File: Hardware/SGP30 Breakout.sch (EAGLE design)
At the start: 26 parts, among them J3 PTH, Q1 MOSFET-NCH-BSS138, Q2 MOSFET-NCH-BSS138, U1 SGP30, U2 MIC5504

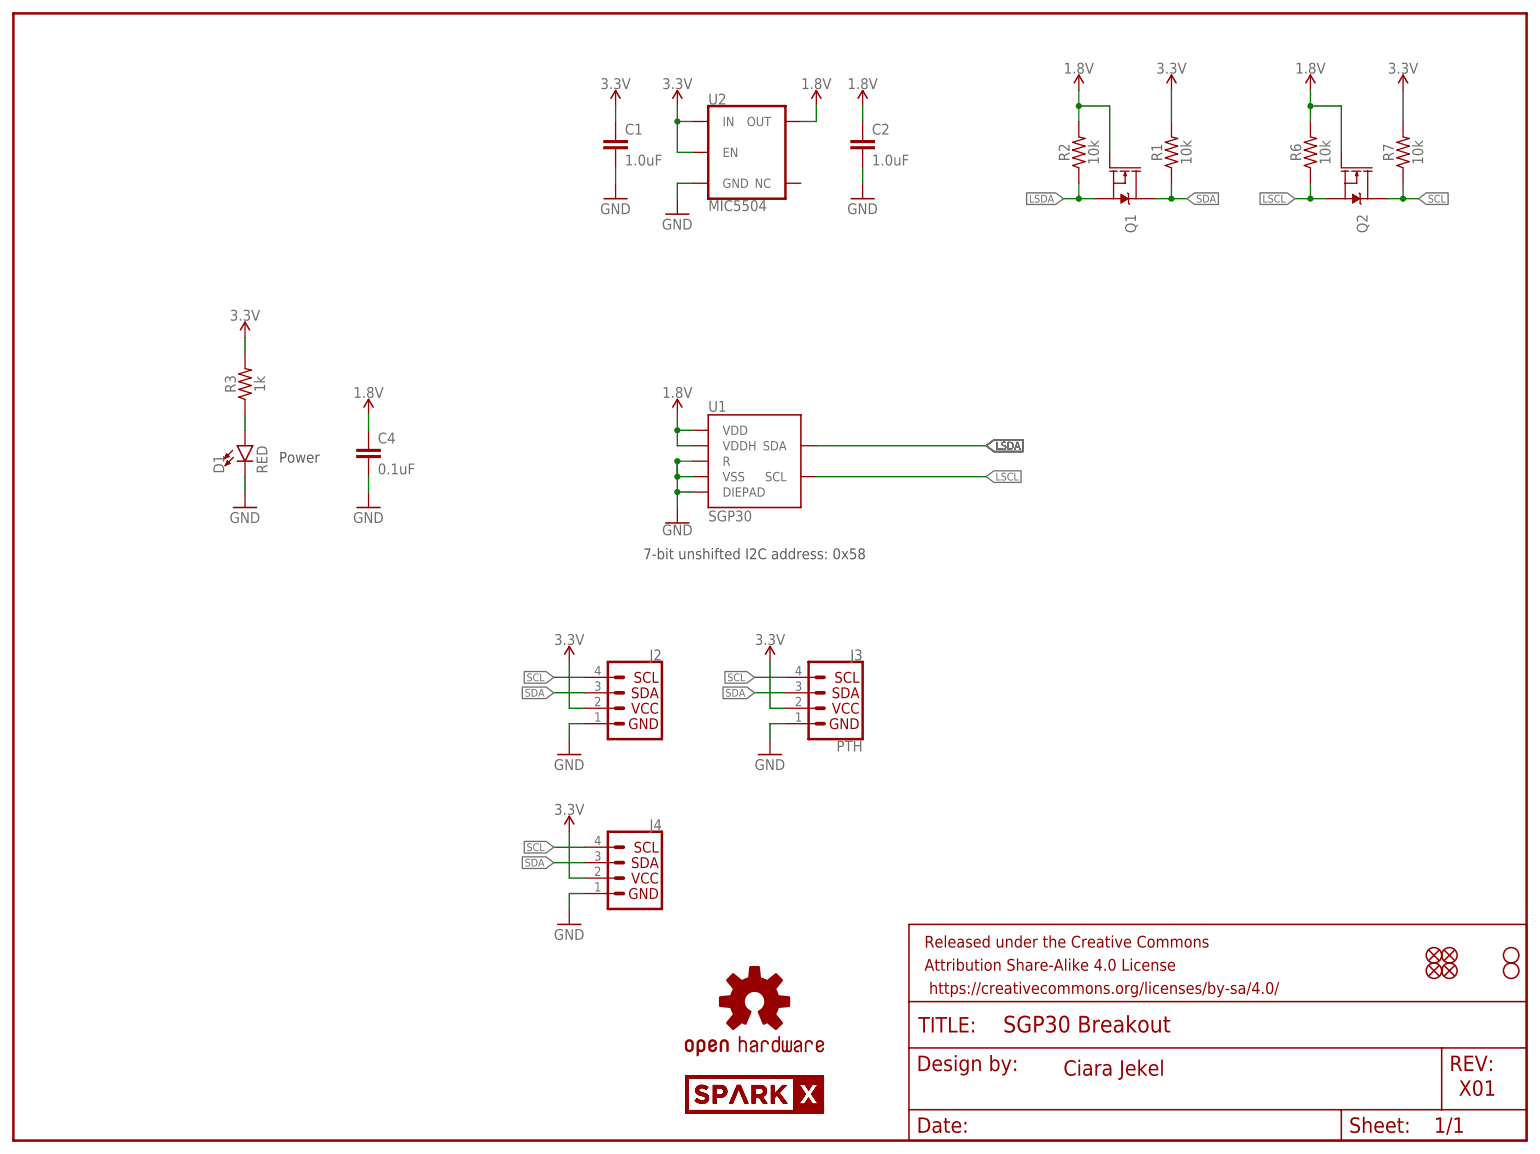
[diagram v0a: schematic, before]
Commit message: added section labels
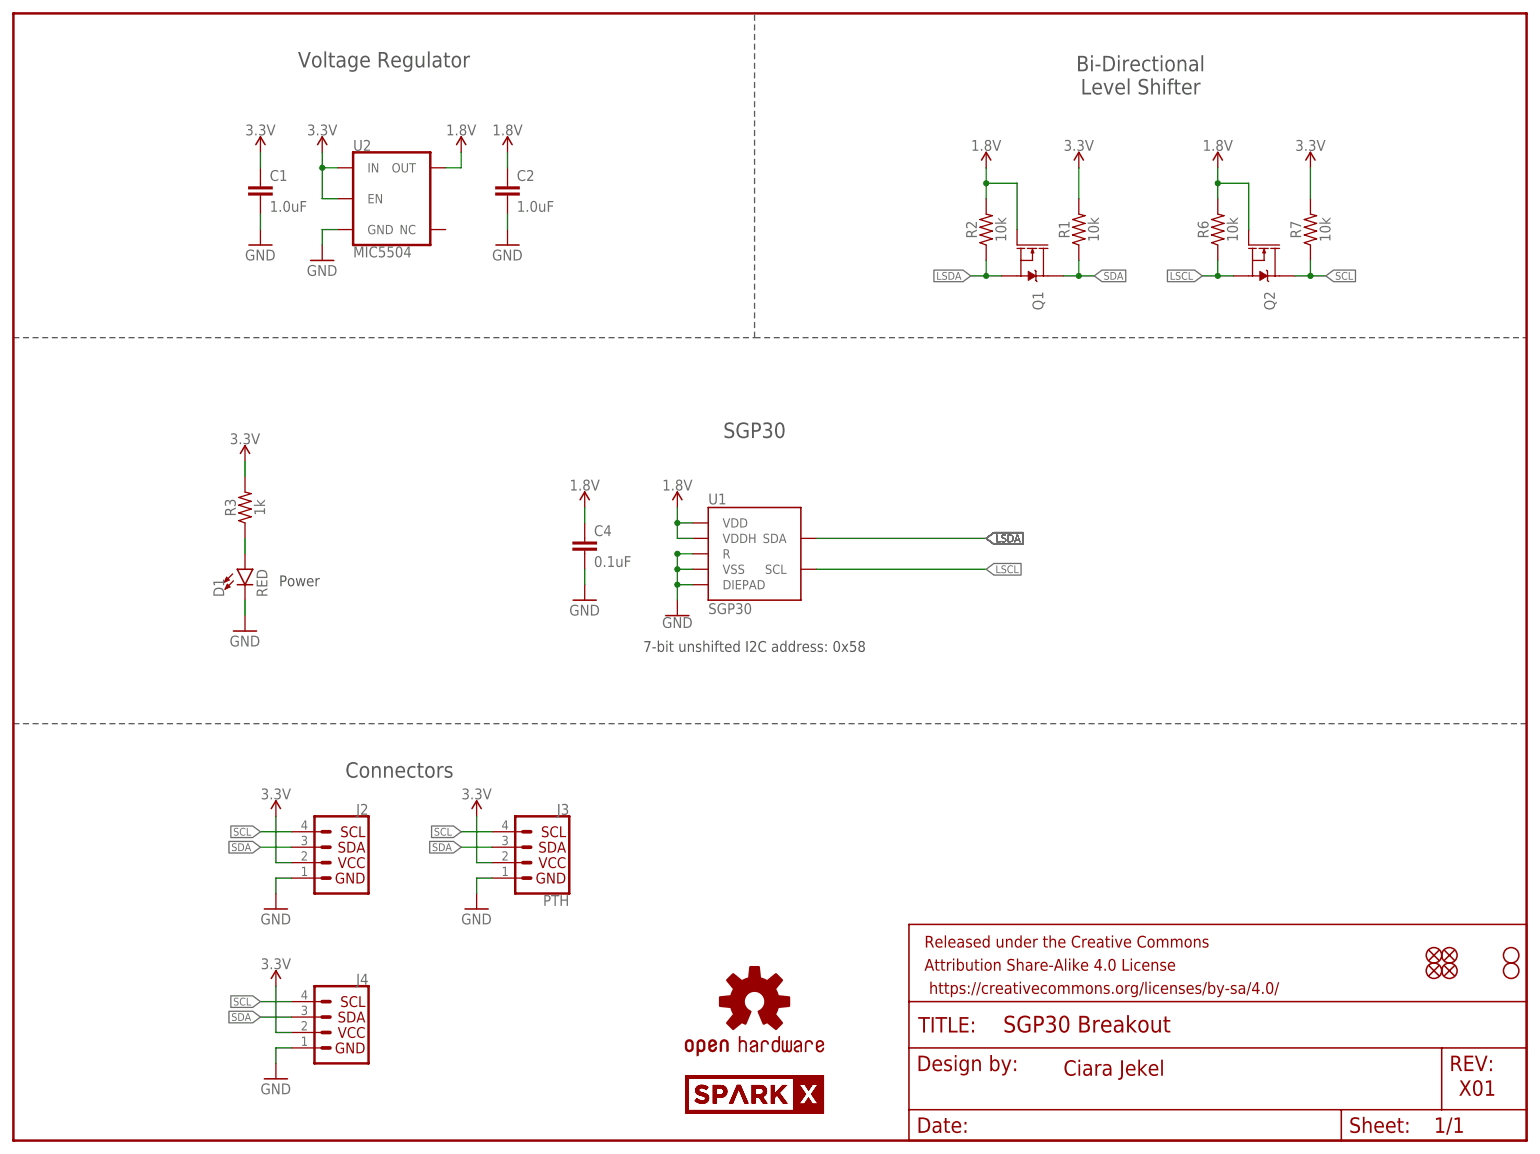
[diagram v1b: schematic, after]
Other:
- note added: "Bi-Directional Level Shifter"
- note added: "Connectors"
- note added: "SGP30"
- note added: "Voltage Regulator"
- moved on the sheet: C1, C2, C4, D1, J2, J3, J4, Q1, Q2, R1, R2, R3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
